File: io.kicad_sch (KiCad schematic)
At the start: 20 parts, among them J1 USB_C_Receptacle_USB2.0_14P, J2 Micro_SD_Card, U3 FT2232HL, Y1 12Mhz

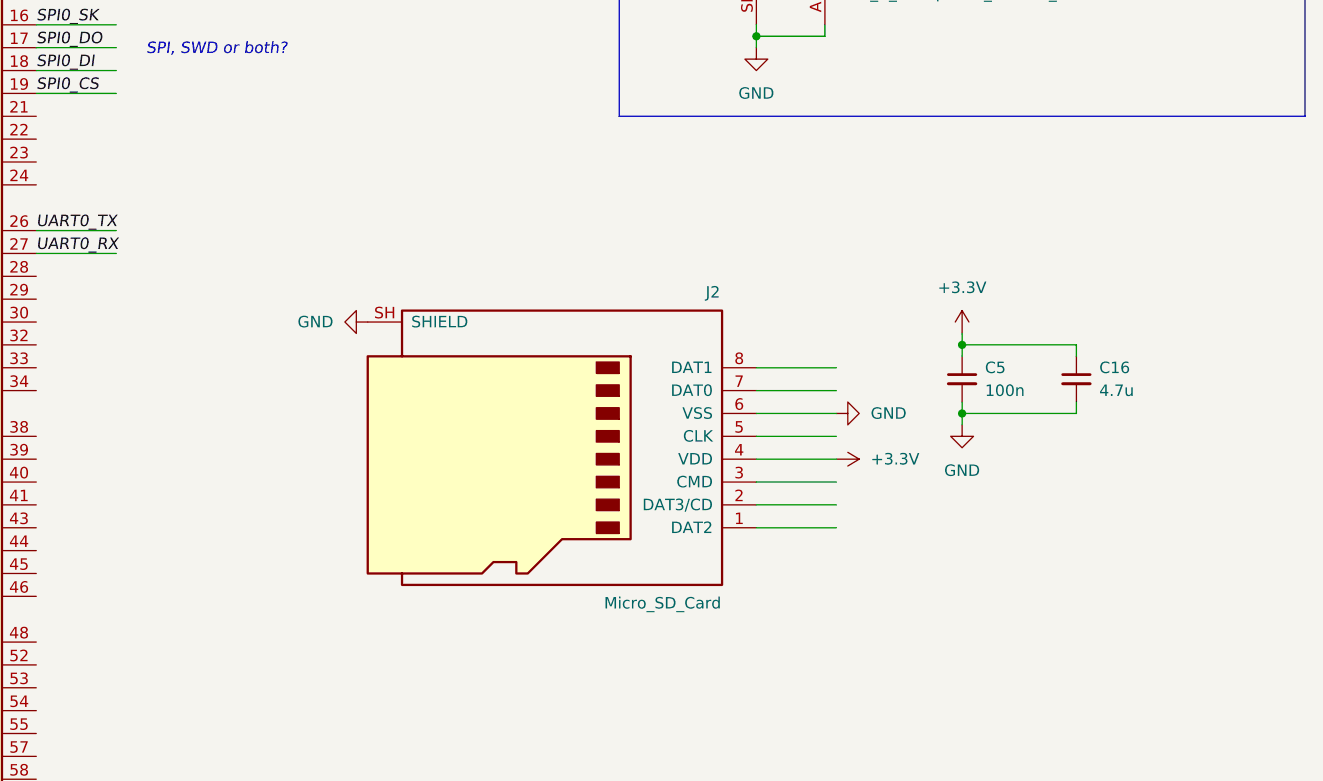
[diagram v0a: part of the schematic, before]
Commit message: MCU wiring
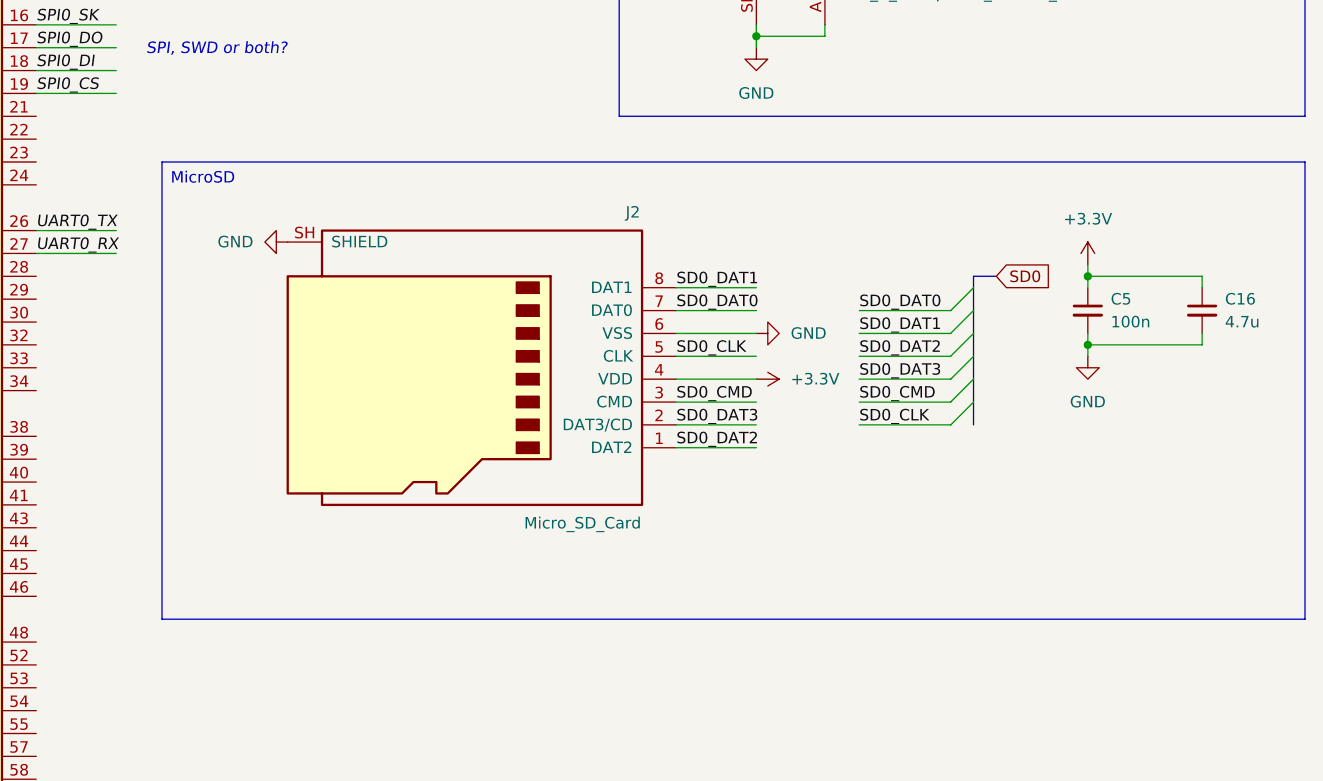
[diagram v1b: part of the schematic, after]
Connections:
- net SD0_DAT2: now reaches J2.1 (DAT2)
- net SD0_DAT3: now reaches J2.2 (DAT3/CD)
- net SD0_CMD: now reaches J2.3 (CMD)
- net SD0_CLK: now reaches J2.5 (CLK)
- net SD0_DAT0: now reaches J2.7 (DAT0)
- net SD0_DAT1: now reaches J2.8 (DAT1)
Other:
- moved on the sheet: C16, C5, J2
